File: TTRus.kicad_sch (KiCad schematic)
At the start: 1 part, among them M1 Module:uaefi/0.2

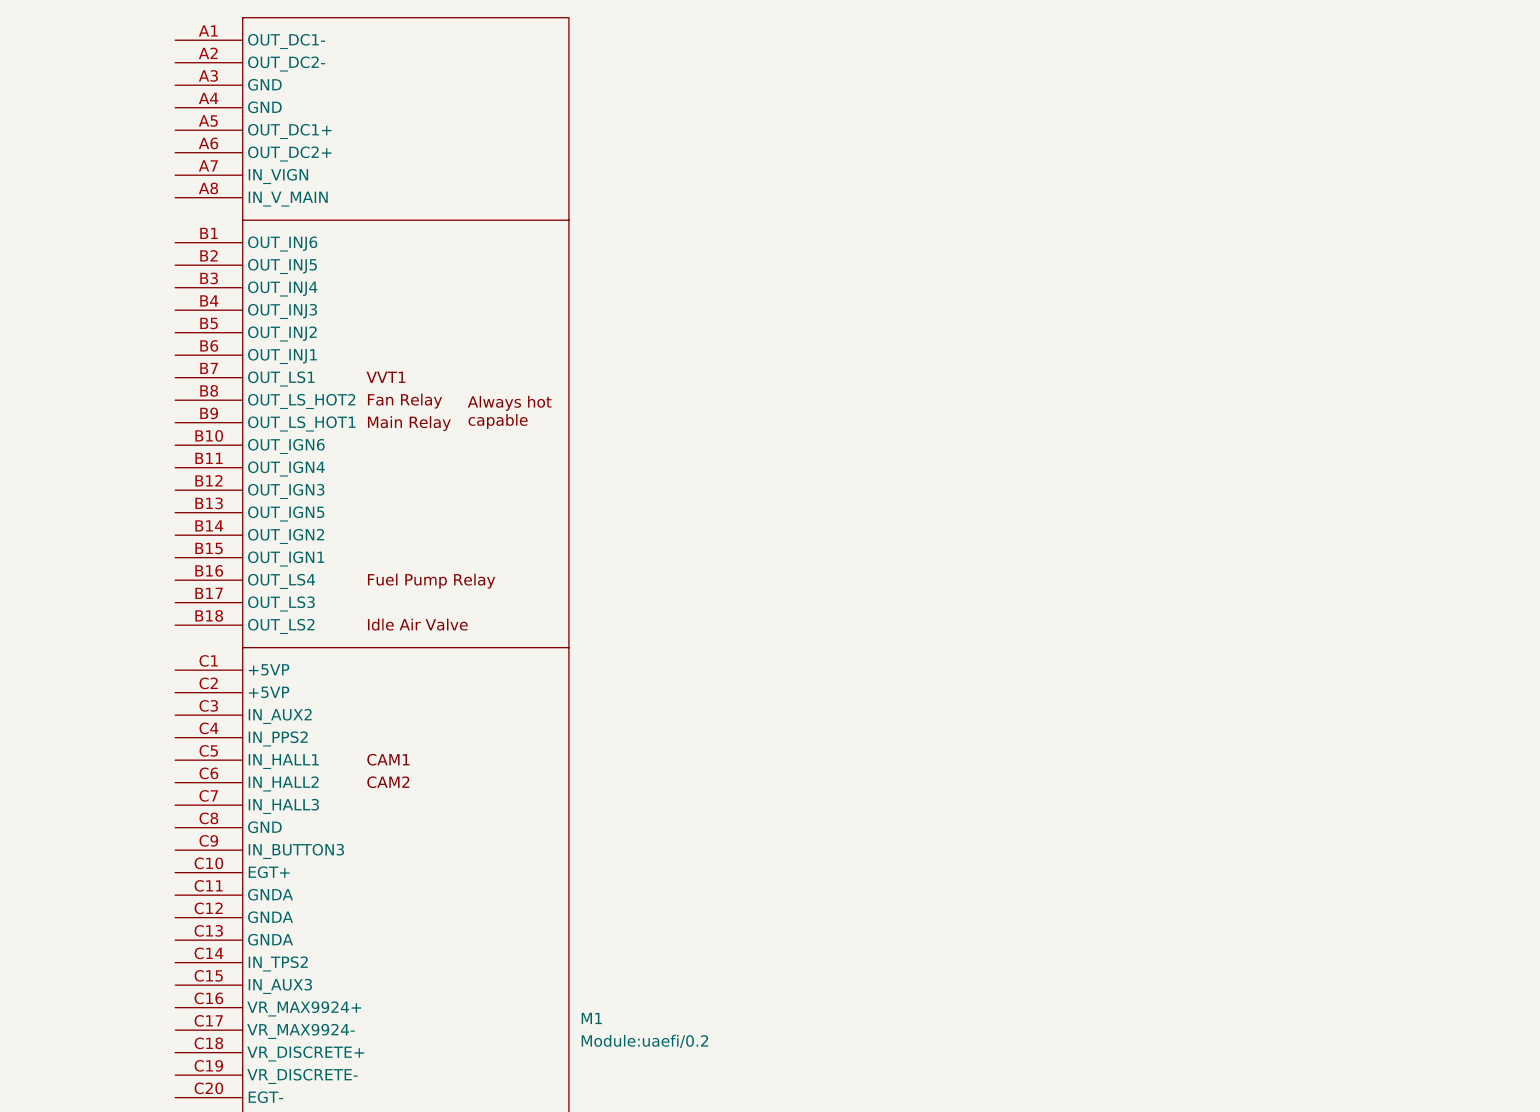
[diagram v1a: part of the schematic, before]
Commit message: Add files via upload
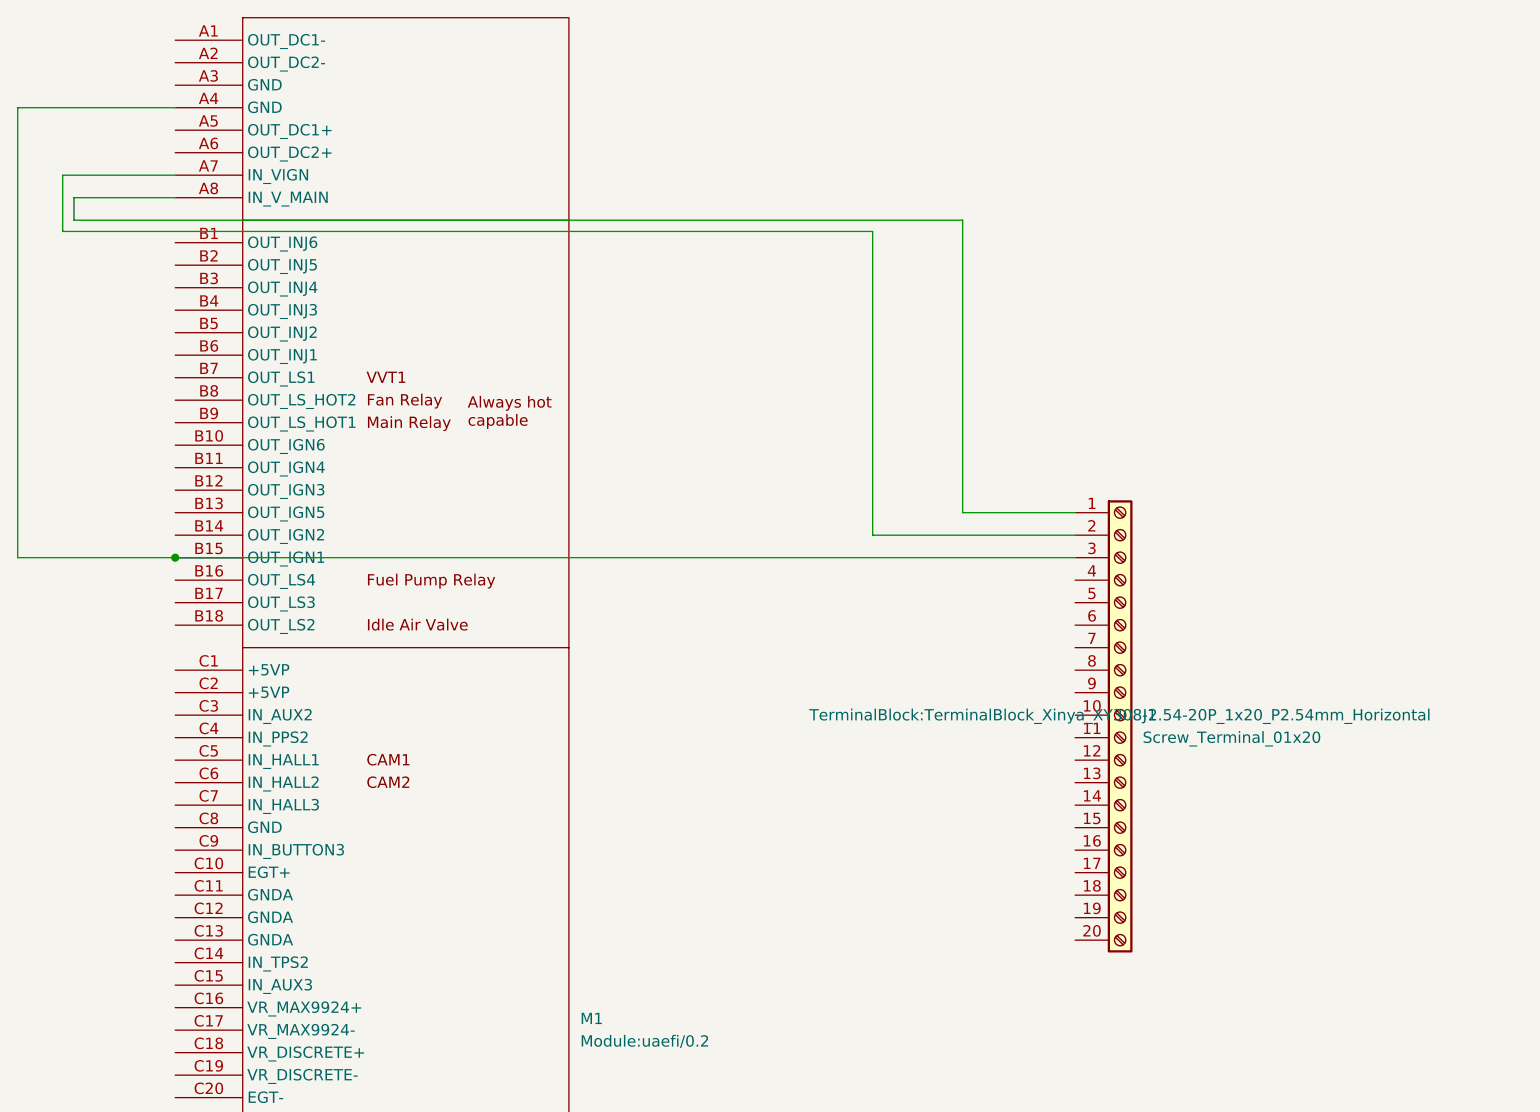
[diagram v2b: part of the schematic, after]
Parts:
- added J1: Screw_Terminal_01x20, TerminalBlock:TerminalBlock_Xinya_XY308-2.54-20P_1x20_P2.54mm_Horizontal, symbol Connector:Screw_Terminal_01x20
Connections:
- net at M1.A4 (GND): now also M1.B15 (OUT_IGN1), J1.3 (Pin_3)
- net at M1.A7 (IN_VIGN): now also J1.2 (Pin_2)
- net at M1.A8 (IN_V_MAIN): now also J1.1 (Pin_1)
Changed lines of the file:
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@@
 	(generator_version "9.0")
 	(paper "A4")
+	(junction
+		(at 48.26 68.58)
+		(diameter 0)
+		(color 0 0 0 0)
+	)
+	(wire
+		(pts
+			(xy 36.83 30.48) (xy 36.83 27.94)
+		)
+		(stroke
+			(width 0)
+			(type default)
+		)
+	)
+	(wire
+		(pts
+			(xy 30.48 17.78) (xy 48.26 17.78)
+		)
+		(stroke
+			(width 0)
+			(type default)
+		)
+	)
+	(wire
+		(pts
+			(xy 127 31.75) (xy 127 66.04)
+		)
+		(stroke
+			(width 0)
+			(type default)
+		)
+	)
+	(wire
+		(pts
+			(xy 149.86 68.58) (xy 48.26 68.58)
+		)
+		(stroke
+			(width 0)
+			(type default)
+		)
+	)
+	(wire
+		(pts
+			(xy 48.26 27.94) (xy 36.83 27.94)
+		)
+		(stroke
+			(width 0)
+			(type default)
+		)
+	)
+	(wire
+		(pts
+			(xy 35.56 31.75) (xy 127 31.75)
+		)
+		(stroke
+			(width 0)
+			(type default)
+		)
+	)
+	(wire
+		(pts
+			(xy 48.26 68.58) (xy 30.48 68.58)
+		)
+		(stroke
+			(width 0)
+			(type default)
+		)
+	)
+	(wire
+		(pts
+			(xy 30.48 68.58) (xy 30.48 17.78)
+		)
+		(stroke
+			(width 0)
+			(type default)
+		)
+	)
+	(wire
+		(pts
+			(xy 137.16 30.48) (xy 36.83 30.48)
+		)
+		(stroke
+			(width 0)
+			(type default)
+		)
+	)
+	(wire
+		(pts
+			(xy 48.26 25.4) (xy 35.56 25.4)
+		)
+		(stroke
+			(width 0)
+			(type default)
+		)
+	)
+	(wire
+		(pts
+			(xy 127 66.04) (xy 149.86 66.04)
+		)
+		(stroke
+			(width 0)
+			(type default)
+		)
+	)
+	(wire
+		(pts
+			(xy 137.16 63.5) (xy 137.16 30.48)
+		)
+		(stroke
+			(width 0)
+			(type default)
+		)
+	)
+	(wire
+		(pts
+			(xy 35.56 25.4) (xy 35.56 31.75)
+		)
+		(stroke
+			(width 0)
+			(type default)
+		)
+	)
+	(wire
+		(pts
+			(xy 149.86 63.5) (xy 137.16 63.5)
+		)
+		(stroke
+			(width 0)
+			(type default)
+		)
+	)
+	(symbol
+		(lib_id "Connector:Screw_Terminal_01x20")
+		(at 154.94 86.36 0)
+		(unit 1)
+		(exclude_from_sim no)
+		(in_bom yes)
+		(on_board yes)
+		(dnp no)
+		(fields_autoplaced yes)
+		(property "Reference" "J1"
+			(at 157.48 86.3599 0)
+			(effects
+				(font
+					(size 1.27 1.27)
+				)
+				(justify left)
+			)
+		)
+		(property "Value" "Screw_Terminal_01x20"
+			(at 157.48 88.8999 0)
+			(effects
+				(font
+					(size 1.27 1.27)
+				)
+				(justify left)
+			)
+		)
+		(property "Footprint" "TerminalBlock:TerminalBlock_Xinya_XY308-2.54-20P_1x20_P2.54mm_Horizontal"
+			(at 154.94 86.36 0)
+			(effects
+				(font
+					(size 1.27 1.27)
+				)
+			)
+		)
+		(property "Datasheet" "~"
+			(at 154.94 86.36 0)
+			(effects
+				(font
+					(size 1.27 1.27)
+				)
+				(hide yes)
+			)
+		)
+		(property "Description" "Generic screw terminal, single row, 01x20, script generated (kicad-library-utils/schlib/autogen/connector/)"
+			(at 154.94 86.36 0)
+			(effects
+				(font
+					(size 1.27 1.27)
+				)
+				(hide yes)
+			)
+		)
+		(pin "8"
+		)
+		(pin "10"
+		)
+		(pin "16"
+		)
+		(pin "19"
+		)
+		(pin "9"
+		)
+		(pin "7"
+		)
+		(pin "18"
+		)
+		(pin "3"
+		)
+		(pin "6"
+		)
+		(pin "13"
+		)
+		(pin "5"
+		)
+		(pin "11"
+		)
+		(pin "4"
+		)
+		(pin "1"
+		)
+		(pin "2"
+		)
+		(pin "12"
+		)
+		(pin "14"
+		)
+		(pin "15"
+		)
+		(pin "17"
+		)
+		(pin "20"
+		)
+		(instances
+			(project ""
+				(path "/7ee6042d-6104-478a-998f-600dea895646"
+					(reference "J1")
+					(unit 1)
+				)
+			)
+		)
+	)
 	(symbol
 		(lib_id "uaefi:Module-uaefi-0.2")
